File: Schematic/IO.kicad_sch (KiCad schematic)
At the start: 78 parts, among them J201 CV1, J202 CV2, J203 CV3, J204 CV4, J205 GATE1, J206 GATE4, J207 GATE2, J208 GATE3, J209 Display, Q101 BC847, SW201 RotaryEncoder_Switch, SW202 RotaryEncoder_Switch, SW203 RotaryEncoder_Switch, SW204 SW_SPST, SW205 SW_SPST, SW206 SW_SPST, SW207 SW_SPST, SW208 SW_SPST, SW209 SW_SPST, U103 MCP4728, U104 TL074, U201 MCP23S17_SO

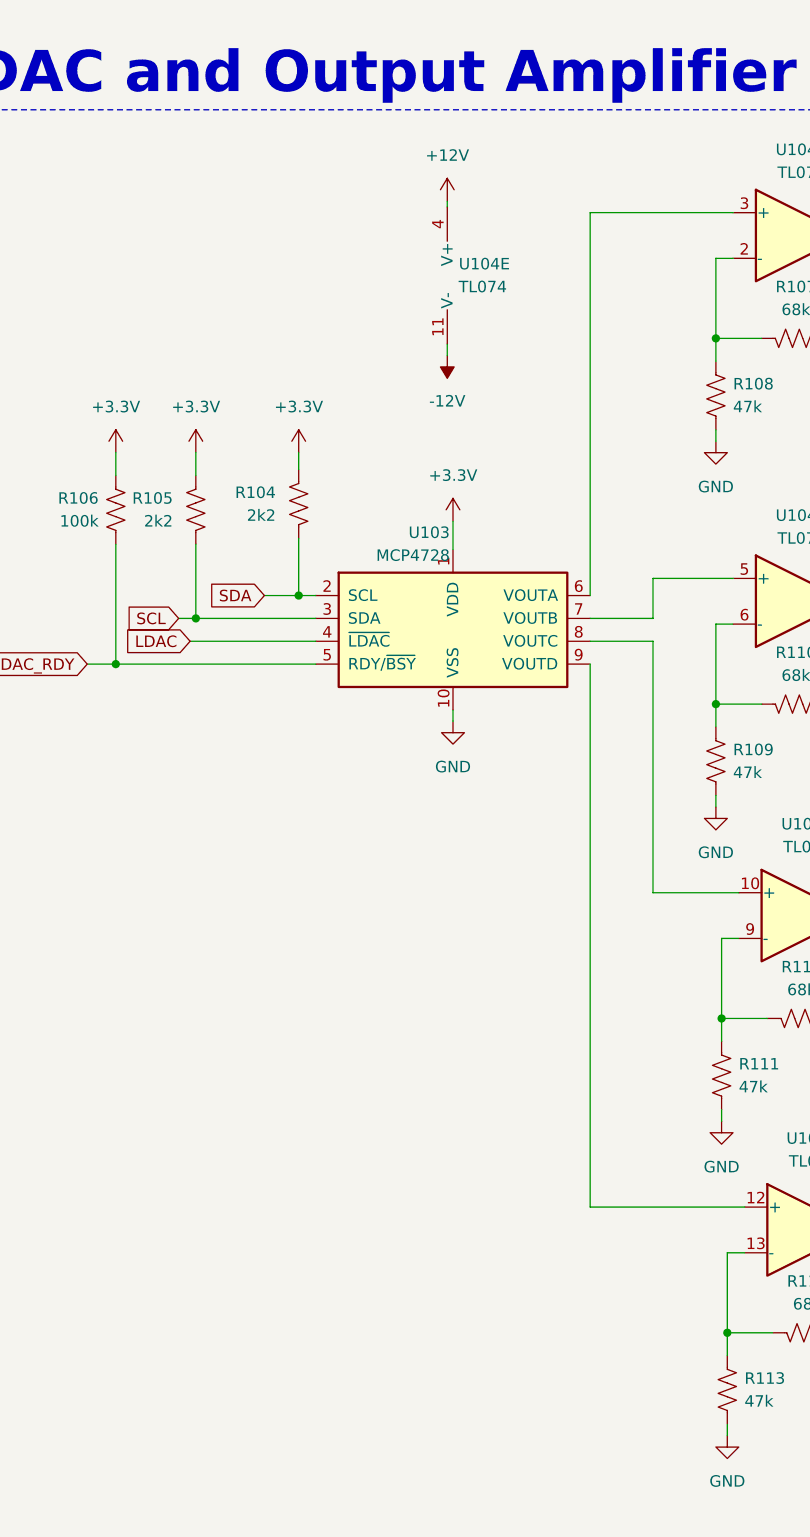
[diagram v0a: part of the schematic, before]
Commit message: PCB in git
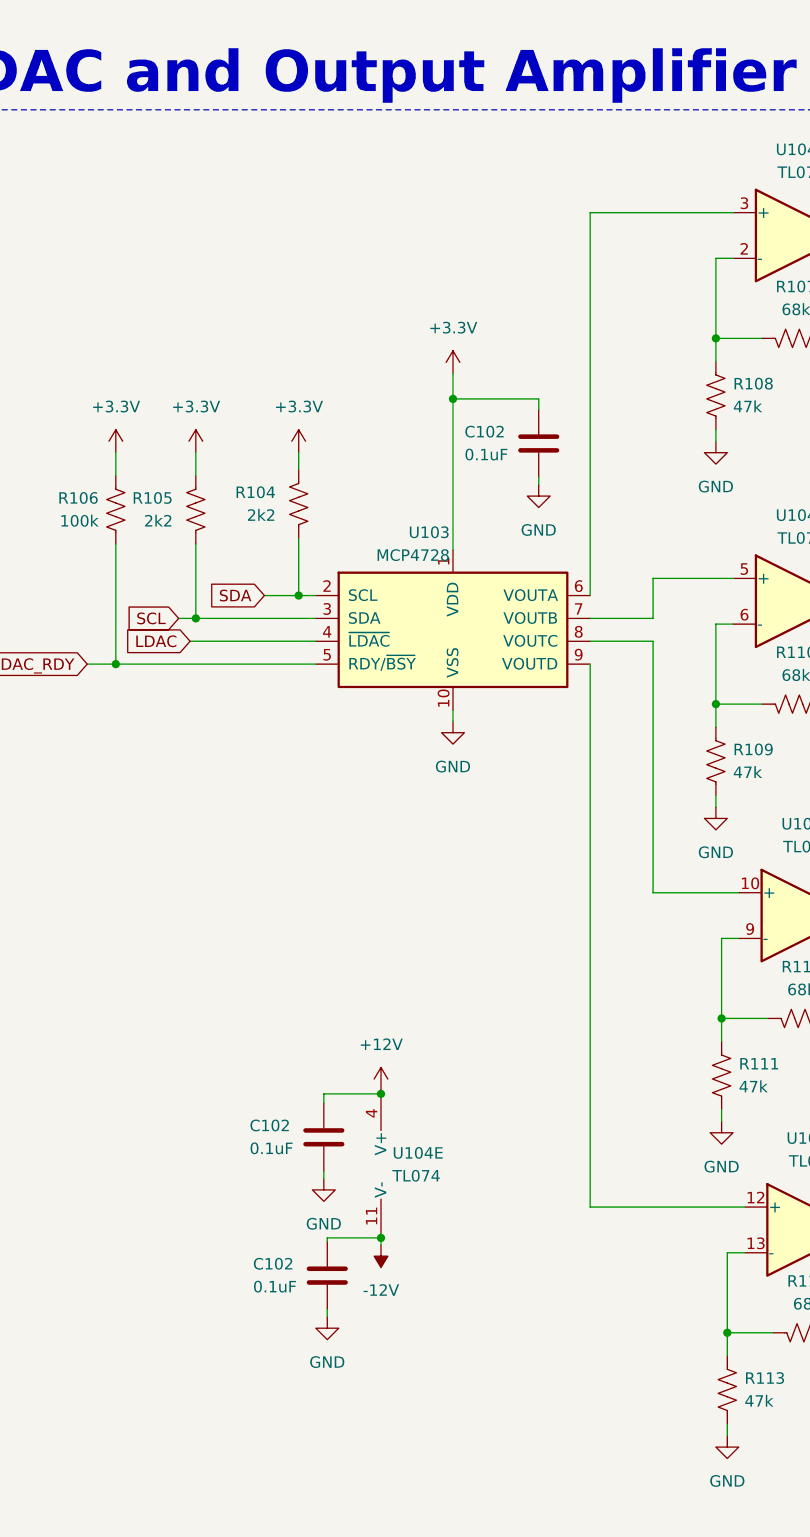
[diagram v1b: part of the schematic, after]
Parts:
- added C102 (x3): 0.1uF, Capacitor_SMD:C_0805_2012Metric, symbol Device:C
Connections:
- net +12V: now also C102.1
- net +3.3V: now also C102.1
- net -12V: now also C102.1
- net GND: now also C102.2, C102.2, C102.2
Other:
- moved on the sheet: U104E
